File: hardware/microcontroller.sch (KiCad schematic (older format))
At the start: 4 parts, among them J1 CONN_02X16, U1 ESP-WROOM-32

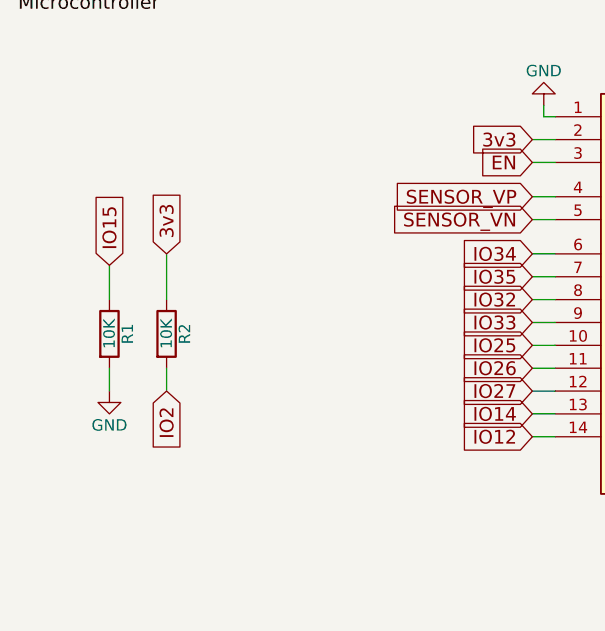
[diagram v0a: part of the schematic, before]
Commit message: update
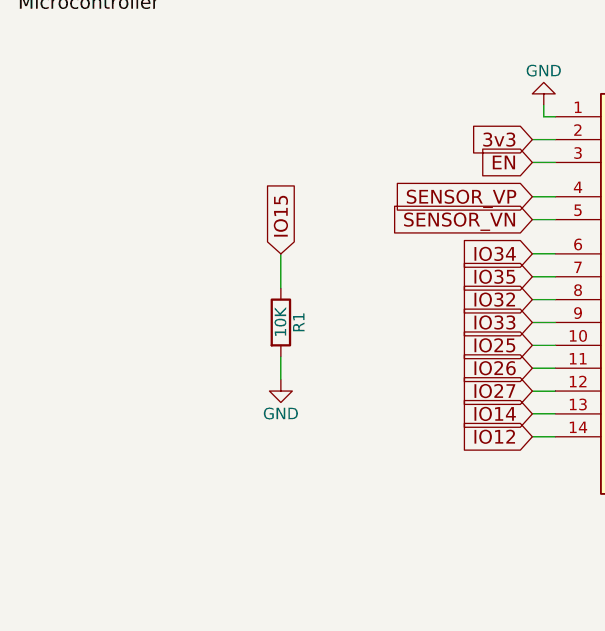
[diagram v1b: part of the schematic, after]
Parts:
- removed R2: 10K, Resistors_SMD:R_0603_HandSoldering, symbol R
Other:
- moved on the sheet: R1
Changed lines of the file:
@@
 EESchema Schematic File Version 2
+LIBS:5v-smart-solar-regulator-rescue
 LIBS:power
 LIBS:device
@@
 LIBS:open-automation
 LIBS:5v-smart-solar-regulator-cache
-EELAYER 25 0
+EELAYER 26 0
 EELAYER END
 $Descr A4 11693 8268
@@
 	-1   0    0    1
 $EndComp
-Text GLabel 2600 3300 1    60   Input ~ 0
+Text GLabel 3350 3250 1    60   Input ~ 0
 IO15
 Text GLabel 5050 4600 3    60   Input ~ 0
@@
 L R R1
 U 1 1 590979AC
-P 2600 3600
-F 0 "R1" V 2680 3600 50  0000 C CNN
-F 1 "10K" V 2600 3600 50  0000 C CNN
-F 2 "Resistors_SMD:R_0603_HandSoldering" V 2530 3600 50  0001 C CNN
-F 3 "http://www.digikey.com/en/resources/datasheets/yageo/rc-series-l-suffix-datasheet" H 2600 3600 50  0001 C CNN
-F 4 "RC0603JR-0710KL" V 2600 3600 60  0001 C CNN "Part Number"
-	1    2600 3600
+P 3350 3550
+F 0 "R1" V 3430 3550 50  0000 C CNN
+F 1 "10K" V 3350 3550 50  0000 C CNN
+F 2 "Resistors_SMD:R_0603_HandSoldering" V 3280 3550 50  0001 C CNN
+F 3 "http://www.digikey.com/en/resources/datasheets/yageo/rc-series-l-suffix-datasheet" H 3350 3550 50  0001 C CNN
+F 4 "RC0603JR-0710KL" V 3350 3550 60  0001 C CNN "Part Number"
+	1    3350 3550
 	1    0    0    -1
 $EndComp
@@
 L GND #PWR02
 U 1 1 590979AD
-P 2600 3850
-F 0 "#PWR02" H 2600 3600 50  0001 C CNN
-F 1 "GND" H 2600 3700 50  0000 C CNN
-F 2 "" H 2600 3850 50  0000 C CNN
-F 3 "" H 2600 3850 50  0000 C CNN
-	1    2600 3850
+P 3350 3800
+F 0 "#PWR02" H 3350 3550 50  0001 C CNN
+F 1 "GND" H 3350 3650 50  0000 C CNN
+F 2 "" H 3350 3800 50  0000 C CNN
+F 3 "" H 3350 3800 50  0000 C CNN
+	1    3350 3800
 	1    0    0    -1
 $EndComp
 Text GLabel 5750 4600 3    60   Input ~ 0
 IO15
-Text GLabel 2850 3850 3    60   Input ~ 0
-IO2
-$Comp
-L R R2
-U 1 1 590979AE
-P 2850 3600
-F 0 "R2" V 2930 3600 50  0000 C CNN
-F 1 "10K" V 2850 3600 50  0000 C CNN
-F 2 "Resistors_SMD:R_0603_HandSoldering" V 2780 3600 50  0001 C CNN
-F 3 "http://www.digikey.com/en/resources/datasheets/yageo/rc-series-l-suffix-datasheet" H 2850 3600 50  0001 C CNN
-F 4 "RC0603JR-0710KL" V 2850 3600 60  0001 C CNN "Part Number"
-	1    2850 3600
-	1    0    0    -1
-$EndComp
-Text GLabel 2850 3250 1    60   Input ~ 0
-3v3
 $Comp
 L ESP-WROOM-32 U1
@@
 	4500 2600 4500 2650
 Wire Wire Line
-	2850 3250 2850 3450
-Wire Wire Line
-	2850 3850 2850 3750
-Wire Wire Line
-	2600 3750 2600 3850
-Wire Wire Line
-	2600 3300 2600 3450
+	3350 3700 3350 3800
+Wire Wire Line
+	3350 3250 3350 3400
 Wire Wire Line
 	4450 4050 4550 4050
